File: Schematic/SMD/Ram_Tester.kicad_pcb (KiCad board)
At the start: 2 copper layers, 38.7 x 59 mm, 35 parts, among them J1 Conn_01x04_Pin, J2 ICSP, J3 USB_C_Receptacle_PowerOnly_6P, Q1 IRLML6402, Q2 IRLML6402, SW1 SW_DIP_x03, SW2 SW_Push, U1 ATmega328-P, U2 RAM / ZIF, U3 ZIP Socket, U4 DIP Socket, Y1 Crystal

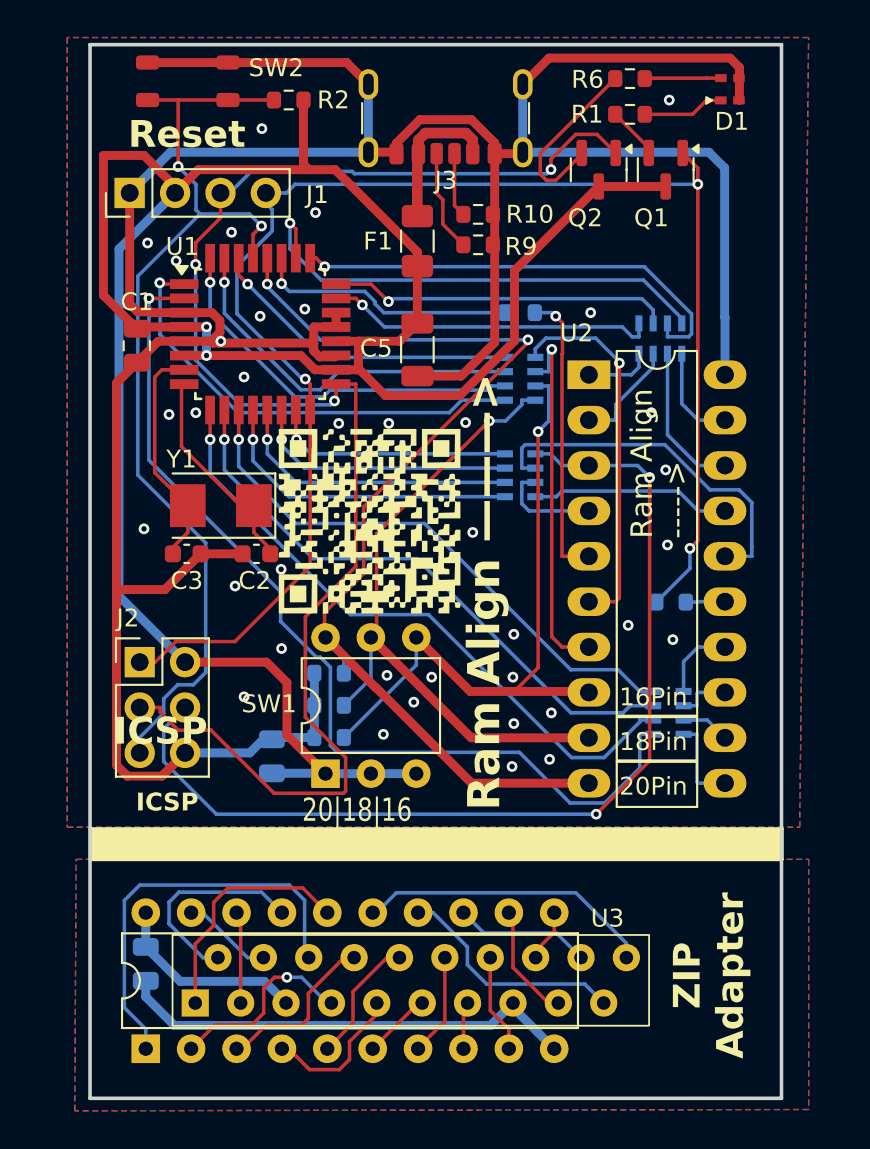
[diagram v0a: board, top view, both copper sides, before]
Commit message: v1.1 of Board
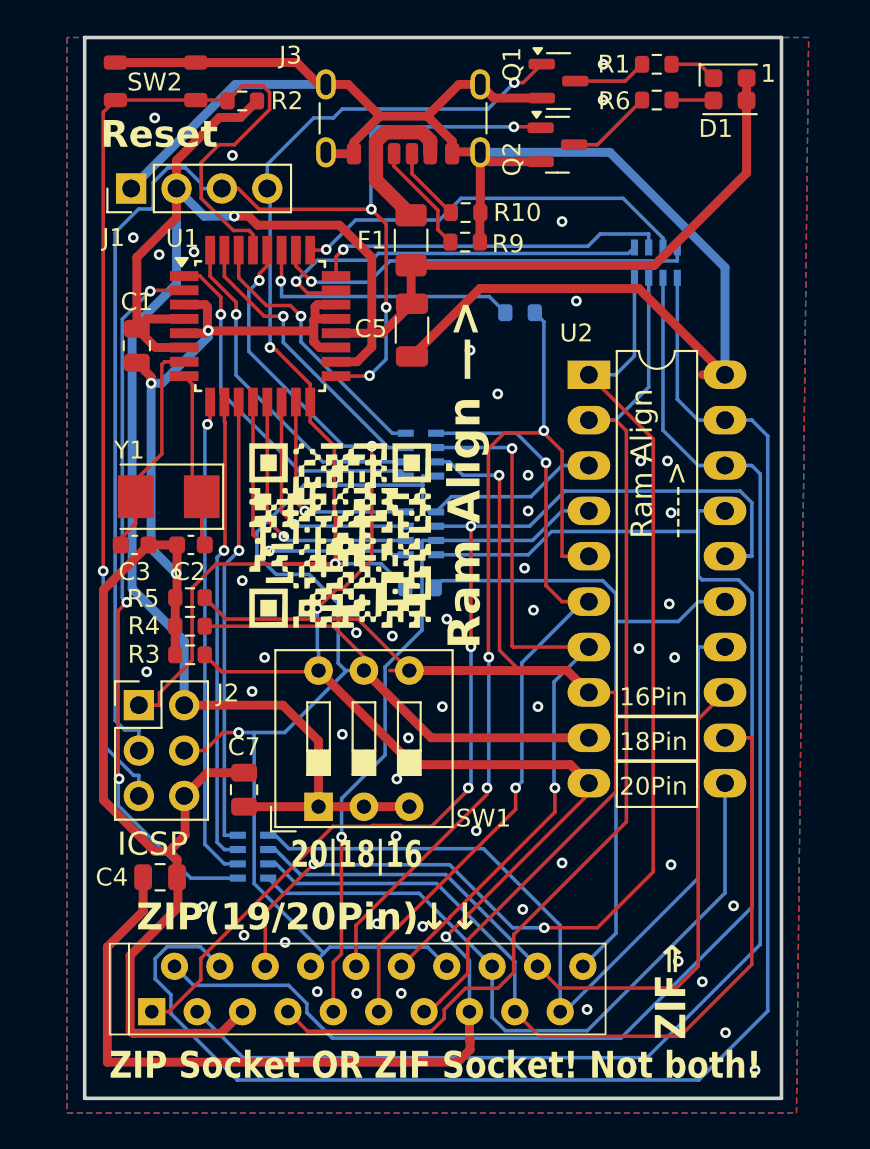
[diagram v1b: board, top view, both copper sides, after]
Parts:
- removed U4: DIP Socket, Package_DIP:DIP-20_W7.62mm
- C4, C7, R3, R4, R5: moved to F.Cu
- D1: value LED_Dual_AAK -> LED_Dual_AAKK; footprint LED_SMD:LED_SMD_RG_AKAK -> LED_SMD:LED_RGB_Wuerth_150080M153000
- Q1, Q2: value IRLML6402 -> BSS138
- SW1: footprint Package_DIP:DIP-6_W7.62mm -> Button_Switch_THT:SW_DIP_SPSTx03_Slide_9.78x9.8mm_W7.62mm_P2.54mm
- moved RN2 24.6 mm to (114.4, 109.8)
- moved R7 14.1 mm to (123.8, 94.8)
- moved R5 11.0 mm to (110.9, 95.3)
- moved R4 8.96 mm to (110.9, 97.0)
- moved R3 7.85 mm to (110.9, 98.5)
- moved Q1 7.79 mm to (131.5, 66.4), turned to 0 degrees
- moved RN3 6.99 mm to (123.8, 87.3)
- moved RN1 6.43 mm to (123.8, 91.8)
- moved C4 4.92 mm to (109.2, 111.0), turned to 180 degrees
- moved RN4 4.26 mm to (136.9, 76.6)
- moved C2 3.70 mm to (110.9, 92.4)
- moved R1 3.18 mm to (137.0, 65.5)
- moved C3 2.96 mm to (107.8, 92.4)
- moved Y1 2.96 mm to (109.7, 89.7)
- moved Q2 2.70 mm to (131.4, 70.0), turned to 0 degrees
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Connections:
- C4 pad 1: /GND2 -> /GND
- C4 pad 2: /5V2 -> Net-(U1-PC5)
- D1 pad 1: Net-(D1-A1) -> /5V
- D1 pad 2: Net-(D1-A2) -> /5V
- D1 pad 3: /GND -> Net-(D1-K1)
- D1 pad 4: /GND -> Net-(D1-K2)
- Q1 pad 2: Net-(Q1-S) -> /GND
- Q1 pad 3: /5V -> Net-(Q1-D)
- Q2 pad 2: Net-(Q2-S) -> /GND
- Q2 pad 3: /5V -> Net-(Q2-D)
- R1 pad 1: Net-(D1-A1) -> Net-(D1-K2)
- R1 pad 2: Net-(Q1-S) -> Net-(Q1-D)
- R4 pad 2: Net-(RN3-R4.1) -> Net-(J2-Pin_4)
- R6 pad 1: Net-(Q2-S) -> Net-(Q2-D)
- R6 pad 2: Net-(D1-A2) -> Net-(D1-K1)
- RN3 pad 4: Net-(RN3-R4.1) -> Net-(J2-Pin_4)
- SW1 pad 5: Net-(RN3-R4.1) -> Net-(J2-Pin_4)
- U2 pad 9: Net-(RN3-R4.1) -> Net-(J2-Pin_4)
- U3 pad 1: Net-(U3-OE) -> Net-(RN1-R2.1)
- U3 pad 10: Net-(U3-N/C) -> Net-(U2-N/C)
- U3 pad 11: Net-(U3-A0) -> Net-(RN3-R1.1)
- U3 pad 12: Net-(U3-A1) -> Net-(RN3-R2.1)
- U3 pad 13: Net-(U3-A2) -> Net-(RN3-R3.1)
- U3 pad 14: Net-(U3-A3) -> Net-(J2-Pin_4)
- U3 pad 15: /5V2 -> Net-(U1-PC5)
- U3 pad 16: Net-(U3-A4) -> Net-(RN2-R4.1)
- U3 pad 17: Net-(U3-A5) -> Net-(RN2-R3.1)
- U3 pad 18: Net-(U3-A6) -> Net-(RN2-R2.1)
- U3 pad 19: Net-(U3-A7) -> Net-(RN2-R1.1)
- U3 pad 2: Net-(U3-CAS) -> Net-(RN1-R4.1)
- U3 pad 20: Net-(U3-A8) -> Net-(U2-A8)
- U3 pad 3: Net-(U3-I/O3) -> Net-(RN4-R2.1)
- U3 pad 4: Net-(U3-I/O4) -> Net-(RN4-R1.1)
- U3 pad 5: /GND2 -> /GND
- U3 pad 6: Net-(U3-I/O1) -> Net-(RN4-R4.1)
- U3 pad 7: Net-(U3-I/O2) -> Net-(RN4-R3.1)
- U3 pad 8: Net-(U3-WE) -> Net-(J2-Pin_4)
- U3 pad 9: Net-(U3-RAS) -> Net-(RN1-R3.1)
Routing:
- net Net-(RN4-R1.1): track 5.60 -> 89.2 mm
- net Net-(RN1-R4.1): track 11.2 -> 81.1 mm
- net Net-(RN4-R2.1): track 8.47 -> 76.5 mm
- net Net-(RN4-R4.1): track 3.73 -> 65.3 mm, vias 0 -> 2
- net Net-(RN4-R3.1): track 6.09 -> 60.3 mm
- net Net-(RN2-R3.1): track 2.73 -> 48.6 mm
- net Net-(U1-PC5): track 60.3 -> 104.9 mm, vias 2 -> 4
- net Net-(RN2-R1.1): track 4.33 -> 48.5 mm
- net Net-(RN1-R2.1): track 20.7 -> 63.3 mm, vias 0 -> 3
- net Net-(RN2-R2.1): track 3.03 -> 43.7 mm
- net Net-(RN3-R4.1): track 37.2 -> 0.00 mm, vias 1 -> 0
- net Net-(J2-Pin_4): track 56.0 -> 93.2 mm, vias 2 -> 1
- net Net-(U2-A8): track 2.21 -> 38.8 mm
- net Net-(RN2-R4.1): track 5.02 -> 40.1 mm
- net Net-(U2-N/C): track 16.4 -> 51.3 mm, vias 1 -> 3
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- removed copper zone on B.Cu, net /GND2
- removed copper zone on F.Cu, net /GND2
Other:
- board size 38.7 x 59 mm -> 39 x 59.4 mm
- board text added: "Ram Align —>"
- board text added: "ZIF⇒"
- board text added: "ZIP Socket OR ZIF Socket! Not both!"
- board text added: "ZIP(19/20Pin)↓↓"
- board text removed: "Lower Side Towards ZIF"
- board text removed: "Ram Align ———>"
- board text removed: "ZIP Adapter"
